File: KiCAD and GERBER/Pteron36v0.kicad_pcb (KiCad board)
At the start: 2 copper layers, 140.1 x 108.1 mm, 56 parts, among them J1 AudioJack4, J2 AudioJack4, J3 Conn_01x04, SW10 SW_PUSH, SW12 SW_PUSH, SW13 SW_PUSH, SW14 SW_PUSH, SW15 SW_PUSH, SW17 SW_PUSH, SW18 SW_PUSH, SW19 SW_PUSH, SW20 SW_PUSH, SW22 SW_PUSH, SW23 SW_PUSH, SW24 SW_PUSH, SW26 SW_PUSH, SW27 SW_PUSH, SW28 SW_PUSH, SW7 SW_PUSH, SW8 SW_PUSH, SW9 SW_PUSH, U1 ProMicro

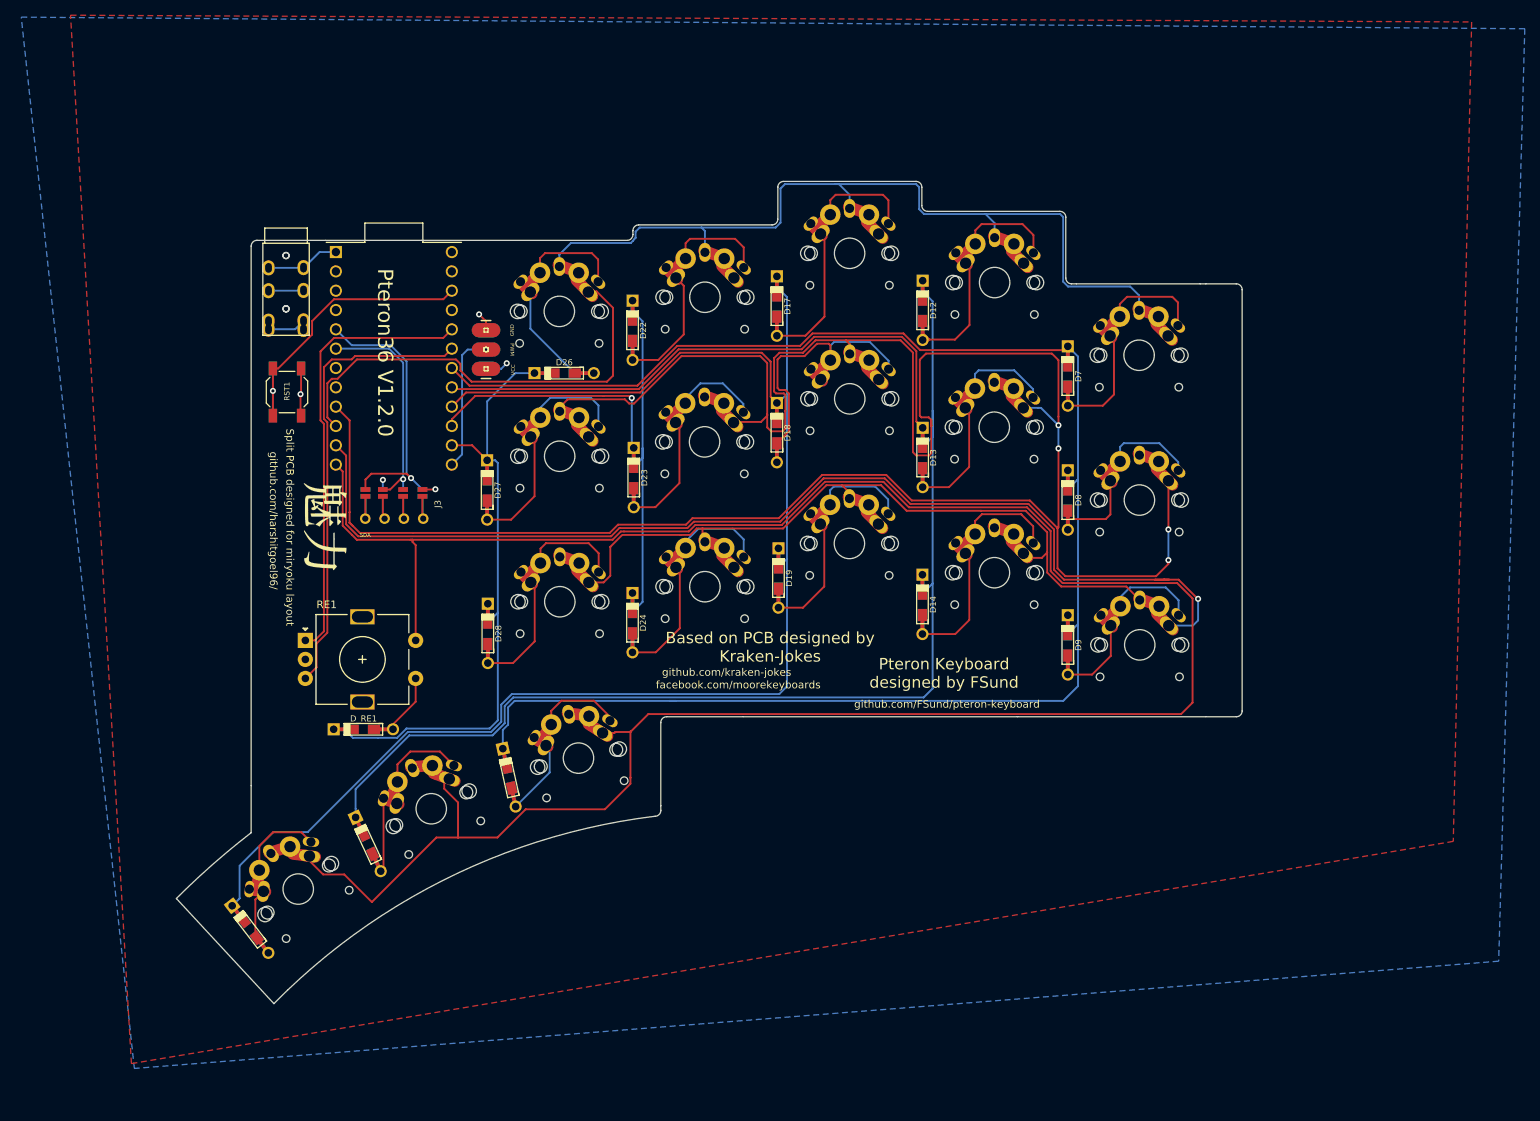
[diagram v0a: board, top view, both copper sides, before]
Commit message: final pcb
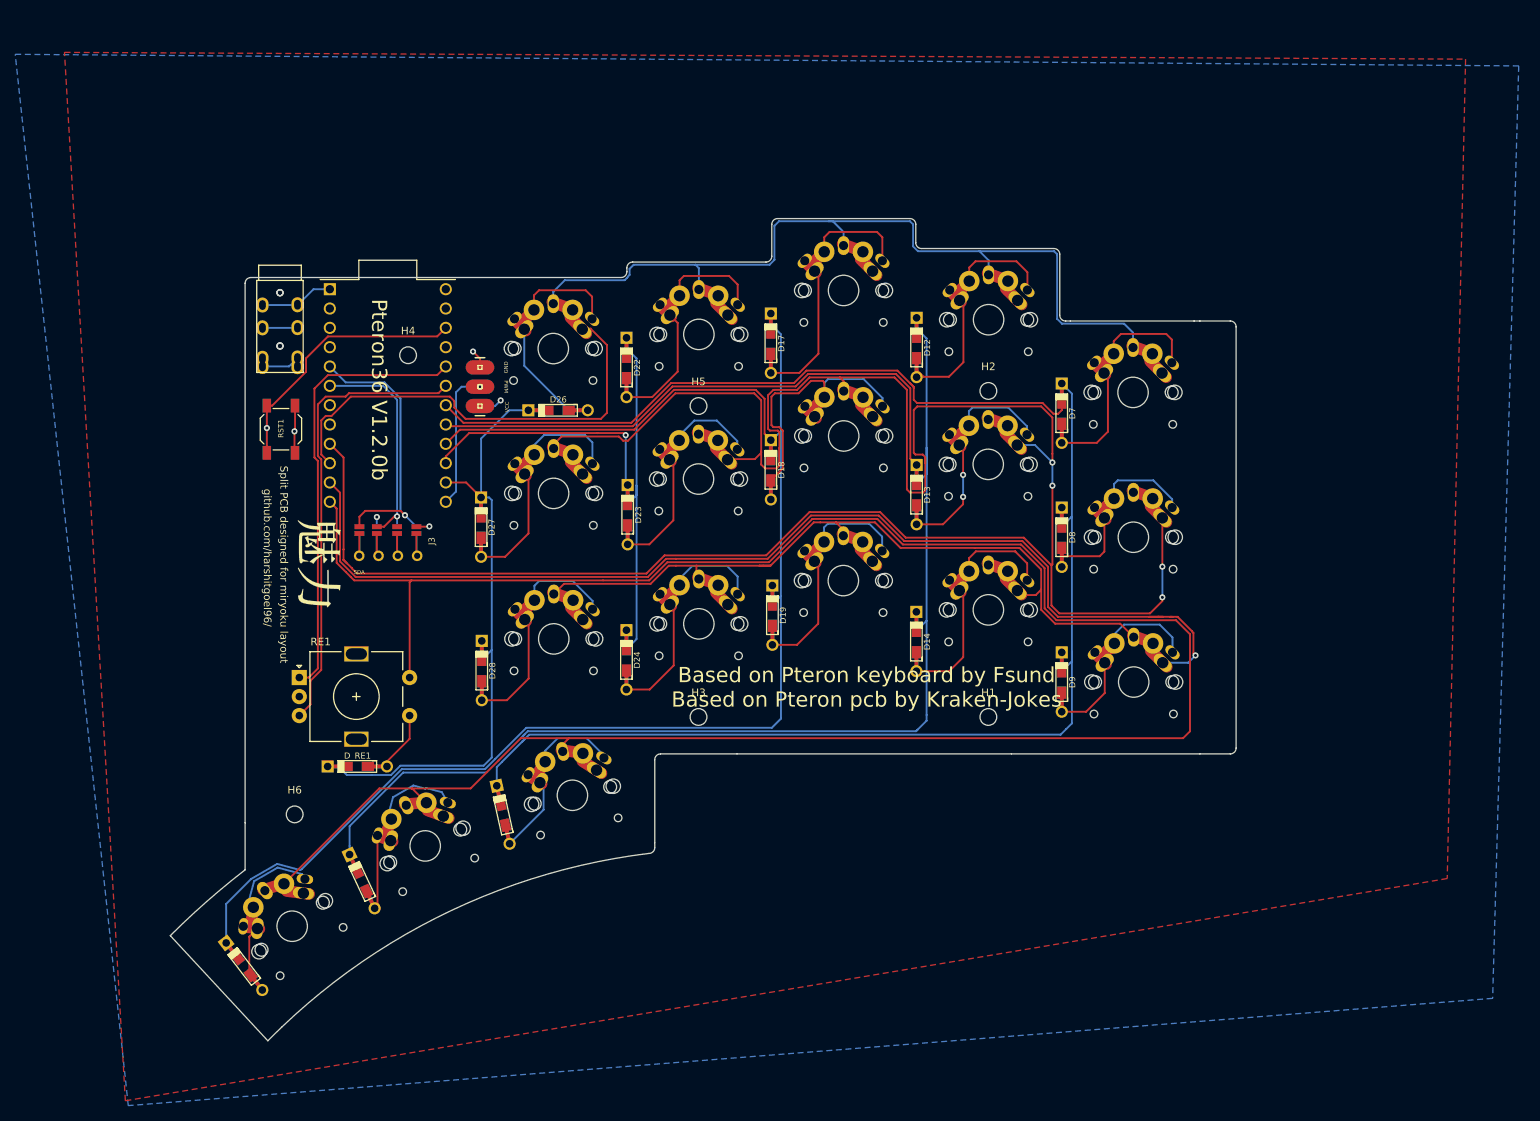
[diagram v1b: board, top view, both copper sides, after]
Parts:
- added H1: MountingHole, MountingHole:MountingHole_2.2mm_M2, F.Cu at (177.8, 106.3)
- added H2: MountingHole, MountingHole:MountingHole_2.2mm_M2, F.Cu at (177.8, 63.5)
- added H3: MountingHole, MountingHole:MountingHole_2.2mm_M2, F.Cu at (139.7, 106.3)
- added H4: MountingHole, MountingHole:MountingHole_2.2mm_M2, F.Cu at (101.5, 58.8)
- added H5: MountingHole, MountingHole:MountingHole_2.2mm_M2, F.Cu at (139.7, 65.5)
- added H6: MountingHole, MountingHole:MountingHole_2.2mm_M2, F.Cu at (86.6, 119.1)
- moved D9 4.95 mm to (187.4, 101.7)
- moved JP2 4.95 mm to (100.1, 81.8)
- moved JP6 4.95 mm to (100.1, 81.8)
- moved U1 4.95 mm to (98.8, 64.1)
- moved SW9 4.95 mm to (196.9, 101.7)
- moved D8 4.95 mm to (187.4, 82.7)
- moved SW8 4.95 mm to (196.8, 82.7)
- moved D14 4.95 mm to (168.3, 96.4)
- moved D20 4.95 mm to (80.0, 139.1)
- moved SW22 4.95 mm to (139.7, 56.0)
- moved JP3 4.95 mm to (97.4, 81.8)
- moved JP4 4.95 mm to (95.1, 81.8)
- moved JP7 4.95 mm to (97.4, 81.8)
- moved JP8 4.95 mm to (95.1, 81.8)
- moved SW19 4.95 mm to (158.7, 88.4)
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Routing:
- net /Row4: track 307.5 -> 292.0 mm
- net /Row3: track 243.4 -> 248.0 mm
- net /Row2: track 306.4 -> 302.5 mm
- net /Col1: track 218.6 -> 222.2 mm
- net Net-(D20-Pad2): track 17.8 -> 19.2 mm
- net /Col2: track 221.5 -> 220.2 mm
- net /Col3: track 197.5 -> 196.5 mm
- net Net-(D28-Pad2): track 29.7 -> 28.9 mm
- net Net-(D13-Pad2): vias 0 -> 2
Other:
- board text added: "Based on Pteron keyboard by Fsund Based on Pteron pcb by Kraken-Jokes"
- board text added: "Pteron36 V1.2.0b"
- board text removed: "Based on PCB designed by Kraken-Jokes"
- board text removed: "Pteron Keyboard designed by FSund"
- board text removed: "Pteron36 V1.2.0"
- board text removed: "facebook.com/moorekeyboards"
- board text removed: "github.com/FSund/pteron-keyboard"
- board text removed: "github.com/kraken-jokes"
